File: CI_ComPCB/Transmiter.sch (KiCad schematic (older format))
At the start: 9 parts, among them J501 RJ45_LED_Shielded, J502 RJ45_LED_Shielded, Q501 Transistor_FET_IRF9540N-CI_Co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, Q502 Transistor_FET_IRF9540N-CI_Co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

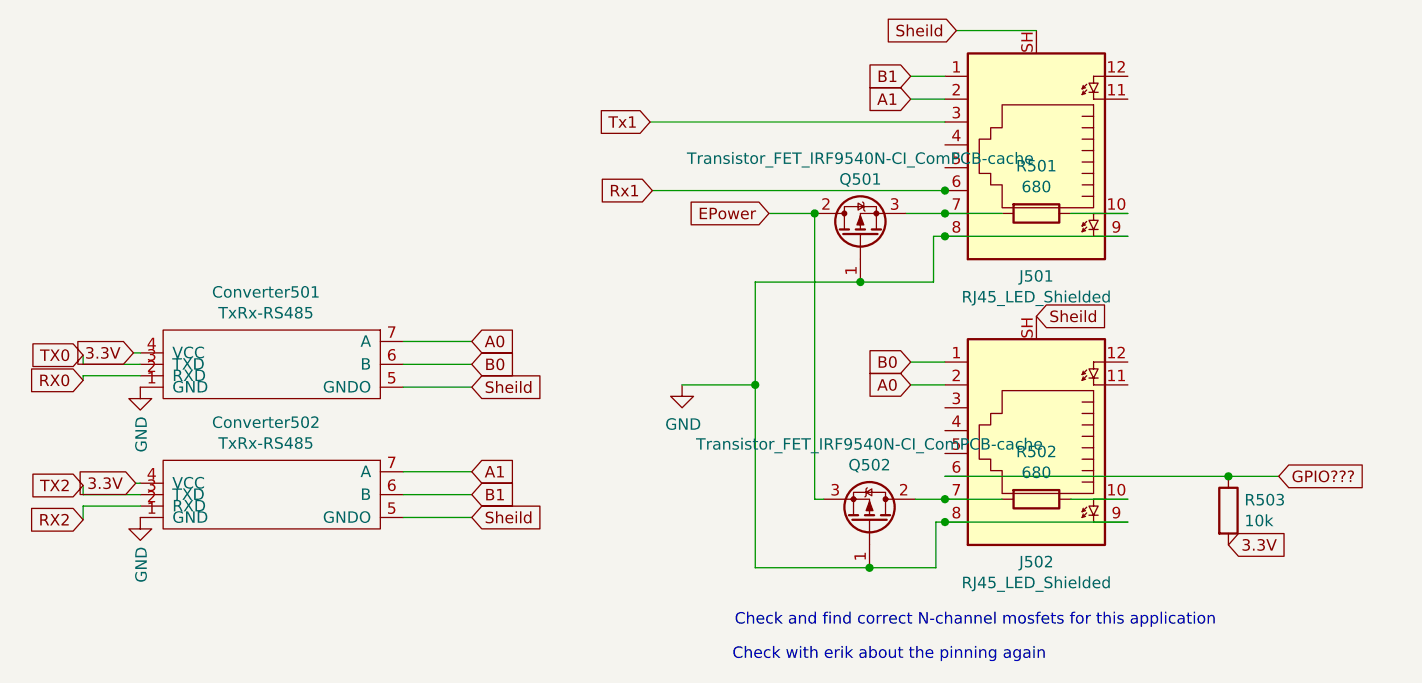
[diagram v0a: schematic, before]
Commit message: switch
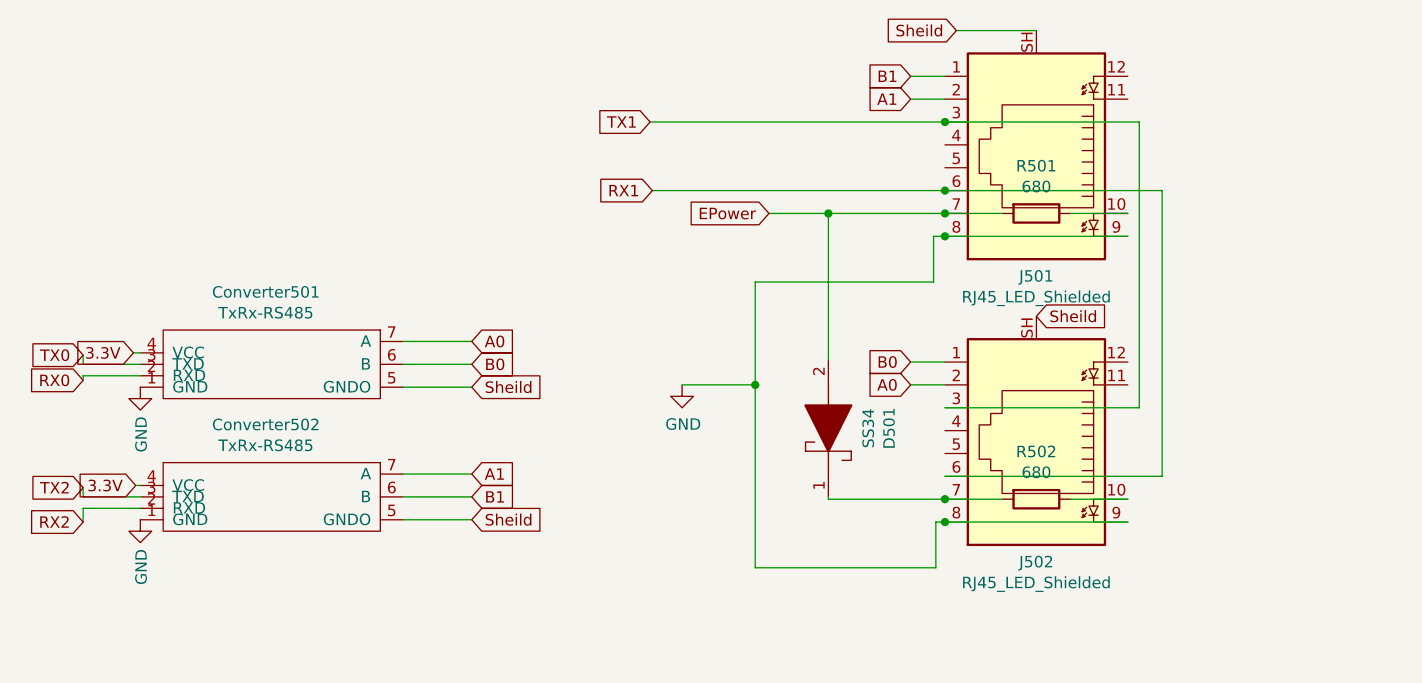
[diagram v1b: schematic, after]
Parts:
- removed Q501, Q502: Transistor_FET_IRF9540N-CI_ComPCB-cache, Package_TO_SOT_THT:TO-220-3_Vertical, symbol CI_ComPCB-rescue:Transistor_FET_IRF9540N-CI_ComPCB-cache
- removed R503: 10k, Resistor_SMD:R_0805_2012Metric, symbol Device:R
- added D501: SS34, digikey-footprints:DO-214AC, symbol CI_ComPCB-rescue:SS34-SamacSys_Parts
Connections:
- net Rx1 is gone; now on net RX1: J501.6
- net Tx1 is gone; now on net TX1: J501.3
- net EPower: now also J501.7, R501.2, D501.2
- net at J502.7, R502.2: now also D501.1
- net TX1: now reaches J502.3
- net GPIO??? renamed RX1
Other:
- note removed: "Check and find correct N-channel mosfets for this application"
- note removed: "Check with erik about the pinning again"
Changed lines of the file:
@@
 L CI_ComPCB-rescue:TxRx-RS485-New_Library-RackComm-rescue-CI_ComPCB-rescue Converter?
 U 1 1 61AB184D
-P 3930 5070
+P 3930 5080
 AR Path="/61AB184D" Ref="Converter?"  Part="1"
 AR Path="/61A9C8FD/61AB184D" Ref="Converter502"  Part="1"
-F 0 "Converter502" H 3880 4355 50  0000 C CNN
-F 1 "TxRx-RS485" H 3880 4446 50  0000 C CNN
-F 2 "CI_ComPCB:TXRX-AB" H 3930 5070 50  0001 C CNN
-F 3 "" H 3930 5070 50  0001 C CNN
-	1    3930 5070
+F 0 "Converter502" H 3880 4365 50  0000 C CNN
+F 1 "TxRx-RS485" H 3880 4456 50  0000 C CNN
+F 2 "CI_ComPCB:TXRX-AB" H 3930 5080 50  0001 C CNN
+F 3 "" H 3930 5080 50  0001 C CNN
+	1    3930 5080
 	1    0    0    1
 $EndComp
-Text GLabel 4780 4570 2    50   Input ~ 0
+Text GLabel 4780 4580 2    50   Input ~ 0
 A1
-Text GLabel 4780 4670 2    50   Input ~ 0
+Text GLabel 4780 4680 2    50   Input ~ 0
 B1
-Text GLabel 4780 4770 2    50   Input ~ 0
-Sheild
-Text GLabel 3310 4620 0    50   Input ~ 0
+Text GLabel 4780 4780 2    50   Input ~ 0
+Sheild
+Text GLabel 3310 4630 0    50   Input ~ 0
 3.3V
 Text GLabel 4780 4200 2    50   Input ~ 0
@@
 	3300 4050 3330 4050
 Wire Wire Line
-	4480 4770 4780 4770
-Wire Wire Line
-	4780 4670 4480 4670
-Wire Wire Line
-	4480 4570 4780 4570
+	4480 4780 4780 4780
+Wire Wire Line
+	4780 4680 4480 4680
+Wire Wire Line
+	4480 4580 4780 4580
 Text GLabel 3080 4170 0    50   Input ~ 0
 RX0
 Wire Wire Line
-	3330 4620 3310 4620
+	3330 4630 3310 4630
 $Comp
 L power:GND #PWR?
 U 1 1 61AB1864
-P 3330 4770
+P 3330 4780
 AR Path="/61AB1864" Ref="#PWR?"  Part="1"
 AR Path="/61A9C8FD/61AB1864" Ref="#PWR0502"  Part="1"
-F 0 "#PWR0502" H 3330 4520 50  0001 C CNN
-F 1 "GND" V 3335 4642 50  0000 R CNN
-F 2 "" H 3330 4770 50  0001 C CNN
-F 3 "" H 3330 4770 50  0001 C CNN
-	1    3330 4770
+F 0 "#PWR0502" H 3330 4530 50  0001 C CNN
+F 1 "GND" V 3335 4652 50  0000 R CNN
+F 2 "" H 3330 4780 50  0001 C CNN
+F 3 "" H 3330 4780 50  0001 C CNN
+	1    3330 4780
 	1    0    0    -1
 $EndComp
@@
 Wire Wire Line
 	3080 4150 3080 4170
-Text GLabel 3080 4630 0    50   Input ~ 0
+Text GLabel 3080 4640 0    50   Input ~ 0
 TX2
-Text GLabel 3080 4780 0    50   Input ~ 0
+Text GLabel 3080 4790 0    50   Input ~ 0
 RX2
 Wire Wire Line
-	3330 4670 3080 4670
-Wire Wire Line
-	3080 4670 3080 4630
-Wire Wire Line
-	3080 4780 3080 4720
-Wire Wire Line
-	3080 4720 3330 4720
+	3330 4680 3080 4680
+Wire Wire Line
+	3080 4680 3080 4640
+Wire Wire Line
+	3080 4790 3080 4730
+Wire Wire Line
+	3080 4730 3330 4730
 Text GLabel 6700 2940 0    50   Input ~ 0
 A1
@@
 Text GLabel 6700 4190 0    50   Input ~ 0
 A0
-Wire Wire Line
-	6080 3440 6280 3440
 Wire Wire Line
 	6850 2840 6700 2840
@@
 	0    1    1    0
 $EndComp
-$Comp
-L CI_ComPCB-rescue:Transistor_FET_IRF9540N-CI_ComPCB-cache Q501
-U 1 1 613180DF
-P 6480 3540
-F 0 "Q501" V 6729 3540 50  0000 C CNN
-F 1 "Transistor_FET_IRF9540N-CI_ComPCB-cache" V 6820 3540 50  0000 C CNN
-F 2 "Package_TO_SOT_THT:TO-220-3_Vertical" H 6680 3465 50  0001 L CIN
-F 3 "" H 6480 3540 50  0001 L CNN
-	1    6480 3540
-	0    -1   -1   0
-$EndComp
 Wire Wire Line
 	6850 3440 7100 3440
-Wire Wire Line
-	6850 3440 6680 3440
 Connection ~ 6850 3440
 Wire Wire Line
@@
 Wire Wire Line
 	6800 3540 6800 3740
-Wire Wire Line
-	6800 3740 6480 3740
 Connection ~ 6850 3540
-$Comp
-L CI_ComPCB-rescue:Transistor_FET_IRF9540N-CI_ComPCB-cache Q502
-U 1 1 6132AA49
-P 6520 4790
-F 0 "Q502" V 6769 4790 50  0000 C CNN
-F 1 "Transistor_FET_IRF9540N-CI_ComPCB-cache" V 6860 4790 50  0000 C CNN
-F 2 "Package_TO_SOT_THT:TO-220-3_Vertical" H 6720 4715 50  0001 L CIN
-F 3 "" H 6520 4790 50  0001 L CNN
-	1    6520 4790
-	0    1    -1   0
-$EndComp
-Wire Wire Line
-	6720 4690 6850 4690
 Connection ~ 6850 4690
 Wire Wire Line
@@
 Wire Wire Line
 	6810 4790 6810 4990
-Wire Wire Line
-	6810 4990 6520 4990
 Wire Wire Line
 	6810 4790 6850 4790
@@
 	6850 4790 7650 4790
 Wire Wire Line
-	6280 3440 6280 4690
-Wire Wire Line
-	6280 4690 6320 4690
-Connection ~ 6280 3440
-Wire Wire Line
-	6520 4990 6020 4990
-Wire Wire Line
 	6020 4990 6020 4190
 Wire Wire Line
 	6020 4190 5700 4190
-Connection ~ 6520 4990
-Wire Wire Line
-	6480 3740 6020 3740
 Wire Wire Line
 	6020 3740 6020 4190
-Connection ~ 6480 3740
 Connection ~ 6020 4190
-Text Notes 5930 5250 0    50   ~ 0
-Check and find correct N-channel mosfets for this application
 Text GLabel 5570 3340 0    50   Input ~ 0
-Rx1
-Wire Wire Line
-	6860 3340 6850 3340
+RX1
 Connection ~ 6850 3340
 Wire Wire Line
 	6850 3340 5570 3340
 Text GLabel 5560 3040 0    50   Input ~ 0
-Tx1
+TX1
 Wire Wire Line
 	6850 3040 5560 3040
-$Comp
-L Device:R R503
-U 1 1 6133BF6C
-P 8090 4740
-F 0 "R503" H 8160 4786 50  0000 L CNN
-F 1 "10k" H 8160 4695 50  0000 L CNN
-F 2 "Resistor_SMD:R_0805_2012Metric" V 8020 4740 50  0001 C CNN
-F 3 "~" H 8090 4740 50  0001 C CNN
-	1    8090 4740
-	1    0    0    -1
-$EndComp
 Wire Wire Line
 	7400 4690 7650 4690
-Text GLabel 8090 4890 2    50   Input ~ 0
-3.3V
-Text GLabel 8310 4590 2    50   Input ~ 0
-GPIO???
-Wire Wire Line
-	8310 4590 8090 4590
-Connection ~ 8090 4590
-Wire Wire Line
-	6850 4590 8090 4590
-Text Notes 5920 5400 0    50   ~ 0
-Check with erik about the pinning again
+Wire Wire Line
+	6850 4590 7800 4590
+Wire Wire Line
+	7800 4590 7800 3340
+Wire Wire Line
+	6850 3340 7800 3340
+Wire Wire Line
+	7700 4290 7700 3040
+Wire Wire Line
+	7700 3040 6850 3040
+Connection ~ 6850 3040
+Wire Wire Line
+	6850 4290 7700 4290
+Wire Wire Line
+	6020 3740 6800 3740
+Wire Wire Line
+	6020 4990 6810 4990
+$Comp
+L CI_ComPCB-rescue:SS34-SamacSys_Parts D?
+U 1 1 614B2CBA
+P 6340 4780
+AR Path="/61A31DC2/614B2CBA" Ref="D?"  Part="1"
+AR Path="/61A9C8FD/614B2CBA" Ref="D501"  Part="1"
+F 0 "D501" H 6740 4513 50  0000 C CNN
+F 1 "SS34" H 6740 4604 50  0000 C CNN
+F 2 "digikey-footprints:DO-214AC" H 6840 4930 50  0001 L CNN
+F 3 "https://componentsearchengine.com/Datasheets/2/SS34.pdf" H 6840 4830 50  0001 L CNN
+F 4 "ON Semi SS34 SMT Schottky Diode, 40V 3A, 2-Pin DO-214AB" H 6840 4730 50  0001 L CNN "Description"
+F 5 "2.56" H 6840 4630 50  0001 L CNN "Height"
+F 6 "512-SS34" H 6840 4530 50  0001 L CNN "Mouser Part Number"
+F 7 "https://www.mouser.co.uk/ProductDetail/ON-Semiconductor-Fairchild/SS34?qs=2ONuHmP%2FXzb3ub11UdFfdQ%3D%3D" H 6840 4430 50  0001 L CNN "Mouser Price/Stock"
+F 8 "ON Semiconductor" H 6840 4330 50  0001 L CNN "Manufacturer_Name"
+F 9 "SS34" H 6840 4230 50  0001 L CNN "Manufacturer_Part_Number"
+	1    6340 4780
+	0    -1   -1   0
+$EndComp
+Wire Wire Line
+	6340 4690 6340 4680
+Wire Wire Line
+	6340 4690 6850 4690
+Wire Wire Line
+	6340 4080 6340 3440
+Wire Wire Line
+	6080 3440 6340 3440
+Wire Wire Line
+	6340 3440 6850 3440
+Connection ~ 6340 3440
 $EndSCHEMATC
